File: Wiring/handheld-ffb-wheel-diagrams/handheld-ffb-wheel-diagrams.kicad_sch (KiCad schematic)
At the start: 18 parts, among them M1 Motor_DC, SW1 SW_Push, SW2 SW_Push, SW3 SW_Push, U1 DRV8871DDA

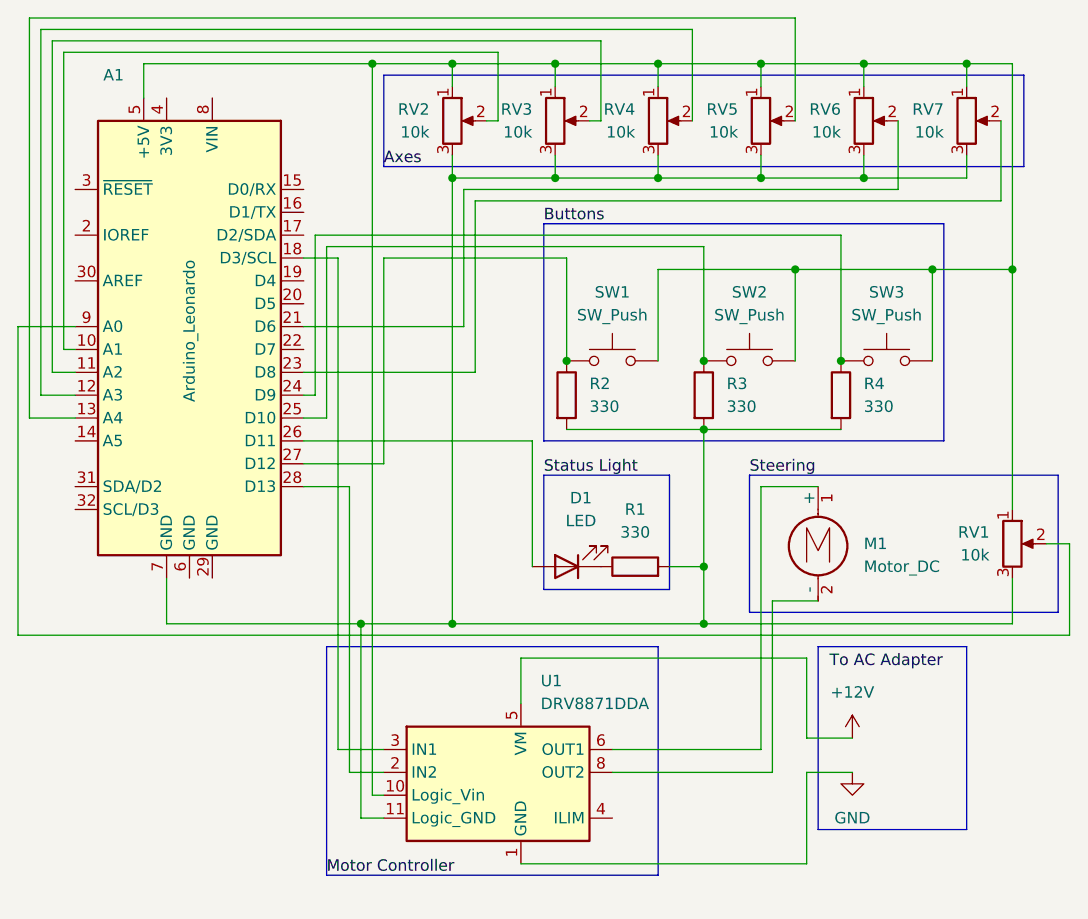
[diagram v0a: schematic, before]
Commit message: Update schematic
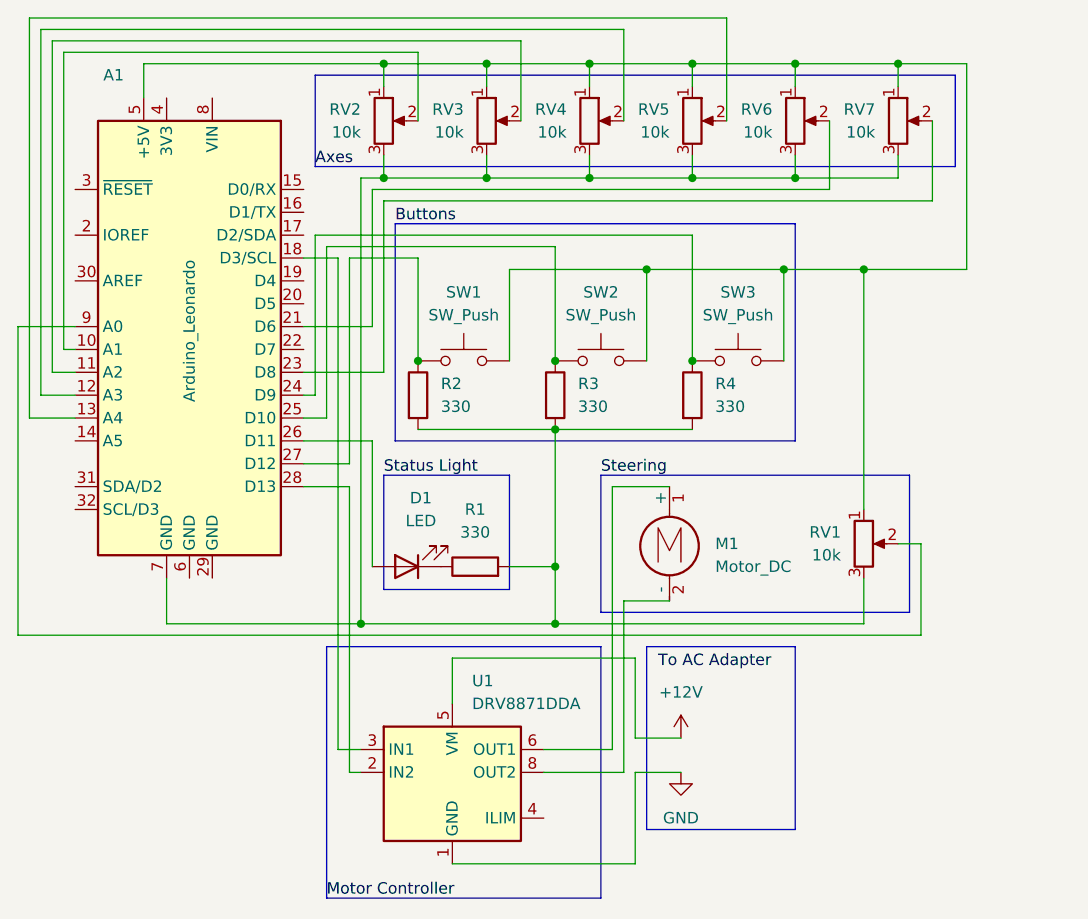
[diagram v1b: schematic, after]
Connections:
- net at A1.5 (+5V), RV1.1, RV2.1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: no longer U1.10 (Logic_Vin)
- net at A1.7 (GND), R1.2, R2.2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: no longer U1.11 (Logic_GND)
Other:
- moved on the sheet: D1, M1, R1, R2, R3, R4, RV1, RV2, RV3, RV4, RV5, RV6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
